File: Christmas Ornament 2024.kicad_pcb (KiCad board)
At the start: 4 copper layers, 76.2 x 76.2 mm, 80 parts, among them J1 USB_B_Micro, J2 Conn_01x03, J3 Conn_01x03, J4 Conn_01x03, J5 Conn_01x03, SW1 PTS815, SW2 PTS815, SW3 PTS815, SW4 PTS815, U1 RP2040, U2 LIS3DH, U3 AMS1117-3.3, U4 W25Q128JVS, U5 TLV61070ADBV, U6 TMP235, Y1 Crystal

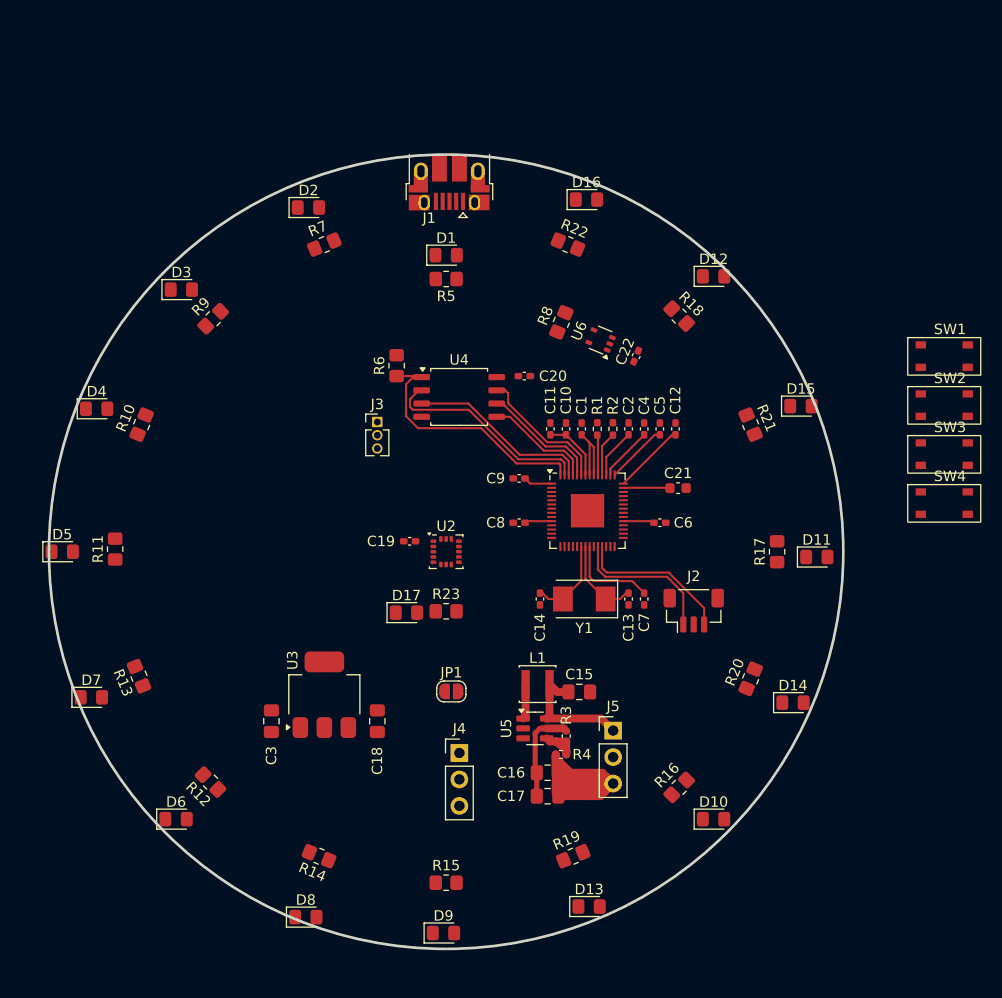
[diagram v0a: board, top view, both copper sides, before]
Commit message: PCB Layout and Routing complete
DRC
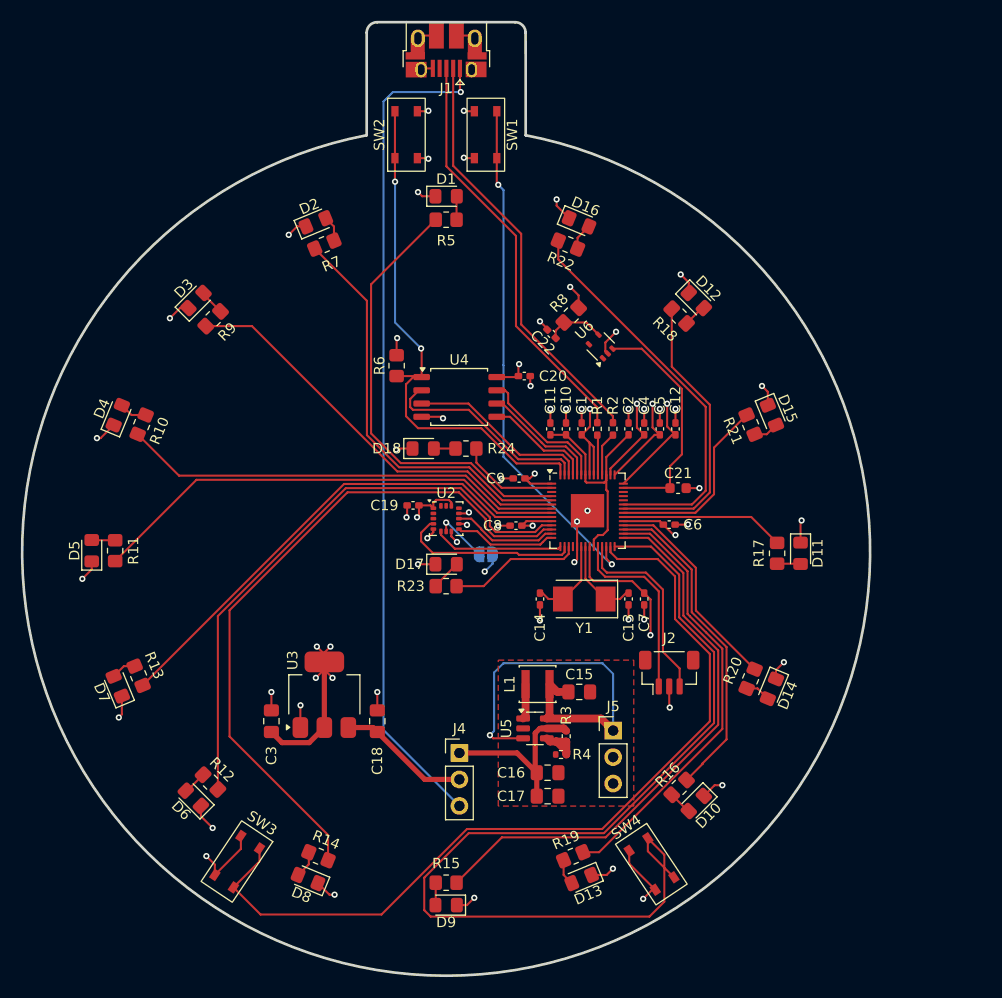
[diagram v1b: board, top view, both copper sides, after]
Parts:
- removed J3: Conn_01x03, Connector_PinHeader_1.27mm:PinHeader_1x03_P1.27mm_Vertical
- added D18: Green LED, LED_SMD:LED_0805_2012Metric_Pad1.15x1.40mm_HandSolder, F.Cu at (124.8, 91.7)
- added R24: 100, Resistor_SMD:R_0805_2012Metric_Pad1.20x1.40mm_HandSolder, F.Cu at (128.9, 91.7)
- JP1: moved to B.Cu
- moved SW3 74.4 mm to (109.1, 130.1), turned to -123.75 degrees
- moved SW2 55.3 mm to (122.1, 63.8), turned to 90 degrees
- moved SW1 46.4 mm to (129.7, 63.8), turned to 90 degrees
- moved SW4 42.3 mm to (146.3, 129.1), turned to -56.25 degrees
- moved JP1 13.6 mm to (130.8, 101.9), turned to 180 degrees
- moved J1 12.8 mm to (127.0, 53.5)
- moved C22 8.41 mm to (137.1, 80.7), turned to 135 degrees
- moved J2 6.40 mm to (148.4, 113.2)
- moved D17 6.01 mm to (127.0, 102.8)
- moved R5 5.69 mm to (127.0, 69.8), turned to 0 degrees
- moved D1 5.65 mm to (127.0, 67.5)
- moved D8 3.66 mm to (113.8, 133.0), turned to 157.5 degrees
- moved C19 3.46 mm to (123.8, 97.2)
- moved U2 3.17 mm to (127.0, 98.4)
- moved D15 2.92 mm to (158.2, 88.5), turned to -67.5 degrees
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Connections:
- U1 pad 3: Net-(J3-Pin_3) -> unconnected-(U1-GPIO1-Pad3)
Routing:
- net BUTTON 2: track 0.00 -> 95.4 mm
- net BUTTON 1: track 0.00 -> 82.2 mm
- net +5V: track 0.00 -> 80.7 mm, vias 0 -> 1
- net LED SSW: track 0.00 -> 66.0 mm
- net GND: track 42.4 -> 102.2 mm, vias 0 -> 52
- net +3V3: track 42.6 -> 100.5 mm, vias 0 -> 19
- net LED SW: track 0.00 -> 56.2 mm
- net LED S: track 0.00 -> 54.5 mm
- net Net-(SW1-A): track 0.00 -> 50.0 mm, vias 0 -> 2
- net LED WSW: track 0.00 -> 48.6 mm
- net LED W: track 0.00 -> 46.4 mm
- net LED N: track 0.00 -> 42.9 mm
- net LED WNW: track 0.00 -> 42.7 mm
- net LED SSE: track 0.00 -> 42.4 mm
- net Net-(J1-D-): track 0.00 -> 40.3 mm
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- added copper zone on In2.Cu, net +3V3
- added copper zone on F.Cu, net GND
- added copper zone on In1.Cu, net GND
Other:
- board size 76.2 x 76.2 mm -> 81.3 x 91.5 mm
- board text added: "To Do: 1. Add mounting holes 2. Top hatched ground pour 3. Silkscreen - Temperature - Christmas Notes - Github Link - Button Labels"
